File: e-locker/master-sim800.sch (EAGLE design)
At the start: 47 parts, among them T1 BC847, T2 BC847, T3 BC847, U1 AT24C128C-SSHM-T, X1 JST-XH-02-PIN-LONG-PAD, X10 JST-XH-05-PIN-LONG-PAD, X11 JST-XH-02-PIN-LONG-PAD, X12 JST-XH-02-PIN-LONG-PAD, X13 JST-XH-02-PIN-LONG-PAD, X2 JST-XH-02-PIN-LONG-PAD, X3 JST-XH-02-PIN-LONG-PAD, X4 JST-XH-02-PIN-LONG-PAD, X5 JST-XH-02-PIN-LONG-PAD, X6 JST-XH-02-PIN-LONG-PAD, X7 JST-XH-04-PIN-LONG-PAD, X8 JST-XH-05-PIN-LONG-PAD, X9 JST-XH-05-PIN-LONG-PAD

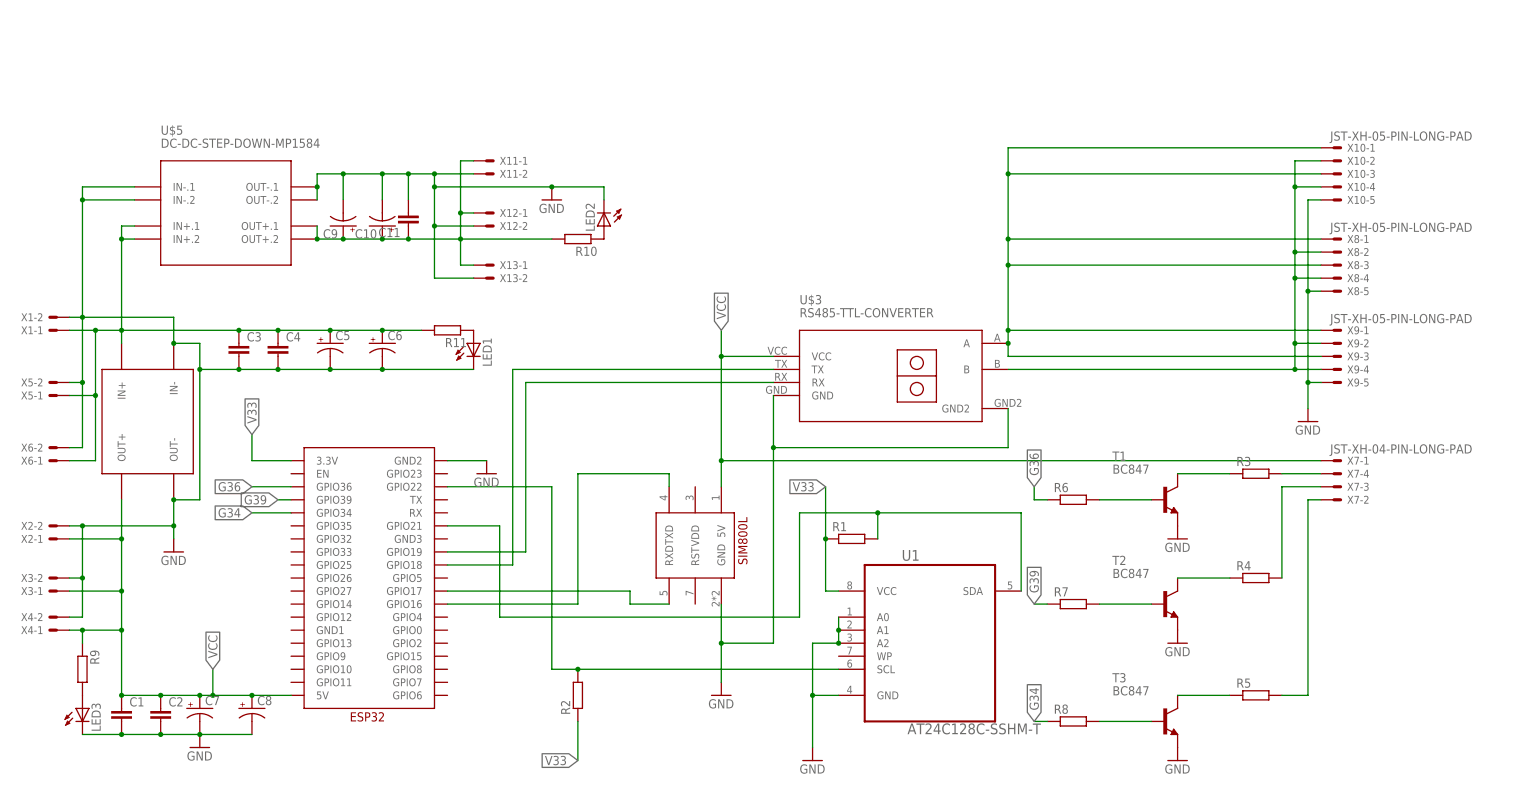
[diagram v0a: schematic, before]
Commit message: master new revision
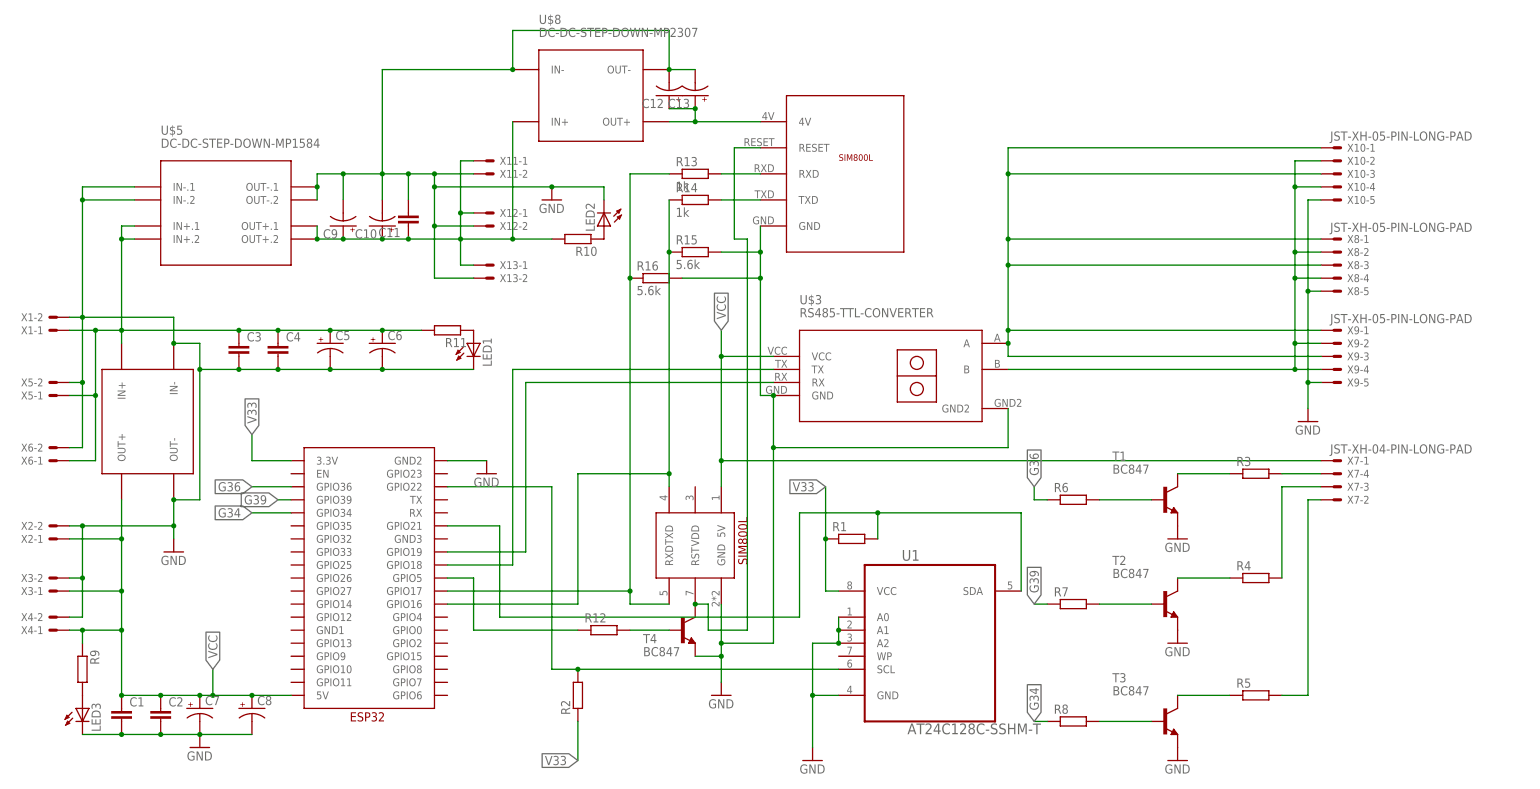
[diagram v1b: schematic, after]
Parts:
- added C12, C13: (no value), adafruit:CPOL-USE5-8.5
- added R12: (no value), eagle-ltspice:RR1206
- added R13, R14: 1k, eagle-ltspice:RR1206
- added R15, R16: 5.6k, eagle-ltspice:RR1206
- added T4: BC847, transistor:BC847
- added U$7: SIM800L-V1, SIM800L:SIM800L-V1
- added U$8: DC-DC-STEP-DOWN-MP2307, diy-modules:DC-DC-STEP-DOWN-MP2307
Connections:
- new net N$18: T4.C, U$2.RST, U$7.RESET
- new net N$24: R12.1, U$1.GPIO5
- new net N$25: R12.2, T4.B
- new net N$26: R13.2, U$7.RXD
- new net N$27: R14.2, U$7.TXD
- new net N$28: C12.+, C13.+, U$7.4V, U$8.OUT+
- net GND: now also C12.-, C13.-, R15.2, R16.2, T4.E, U$7.GND, U$8.IN-, U$8.OUT-
- net N$23: now also U$8.IN+
- net N$3: now also R14.1, R15.1
- net N$4: now also R13.1, R16.1
